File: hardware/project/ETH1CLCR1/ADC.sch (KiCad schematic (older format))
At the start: 103 parts, among them Q1101 BC847W, Q1102 BC847W, Q1103 BC847W, Q1104 BC847W, U1101 ADG419BR, U1102 ADG419BR, U1103 ADR4525BRZ, U1104 ADA4807-2ARM, U1106 AD7380, U1106 ADA4807-2ARM, U1107 ADA4807-1AKSZ-R2, U1108 LT6350, U1109 LT6350, U1110 OPA602, U1111 OPA602, U1112 PGA103, U1113 PGA103

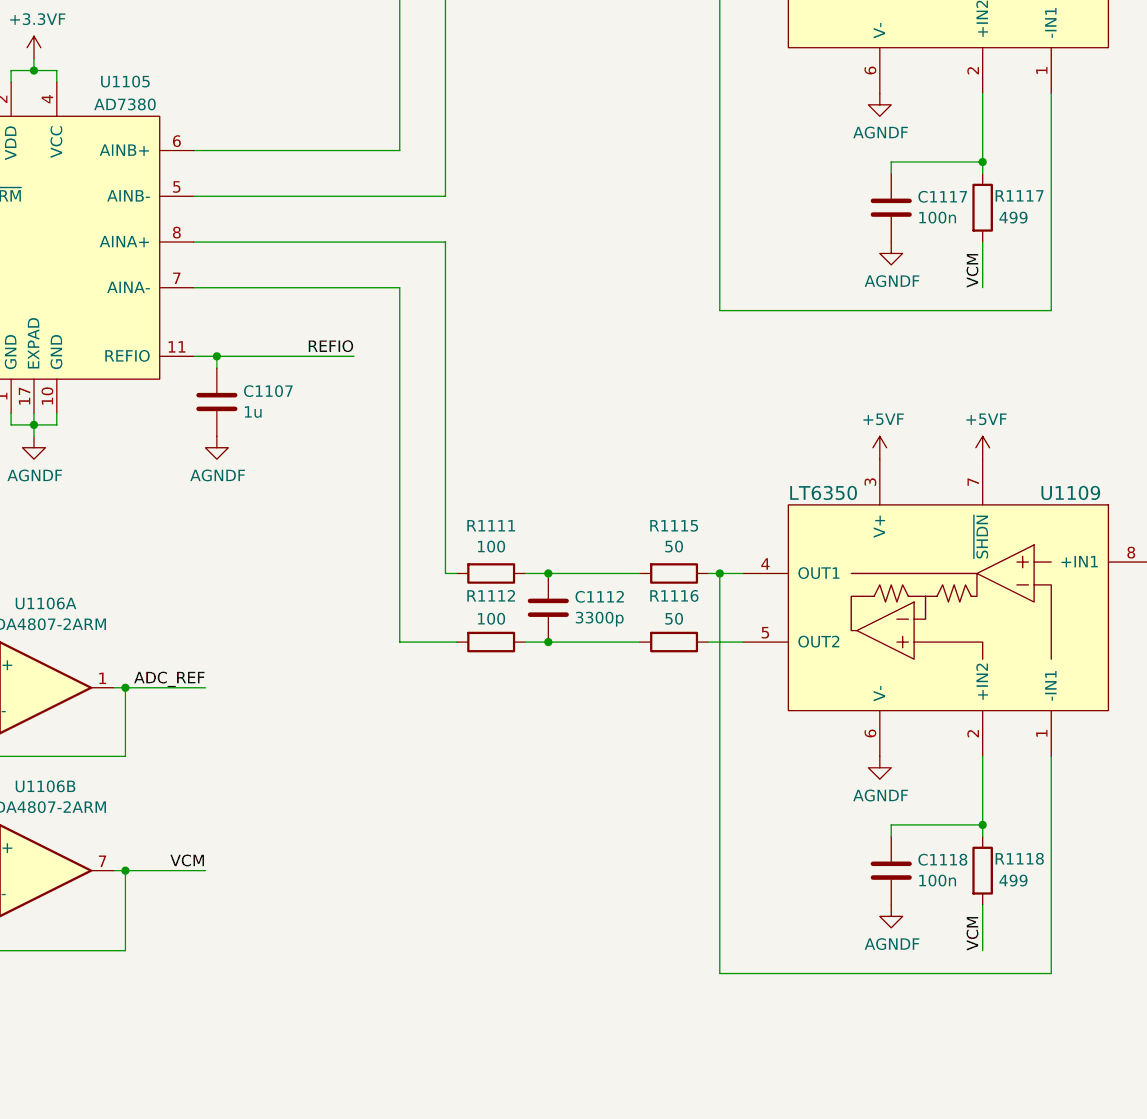
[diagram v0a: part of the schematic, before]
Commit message: PCB done.
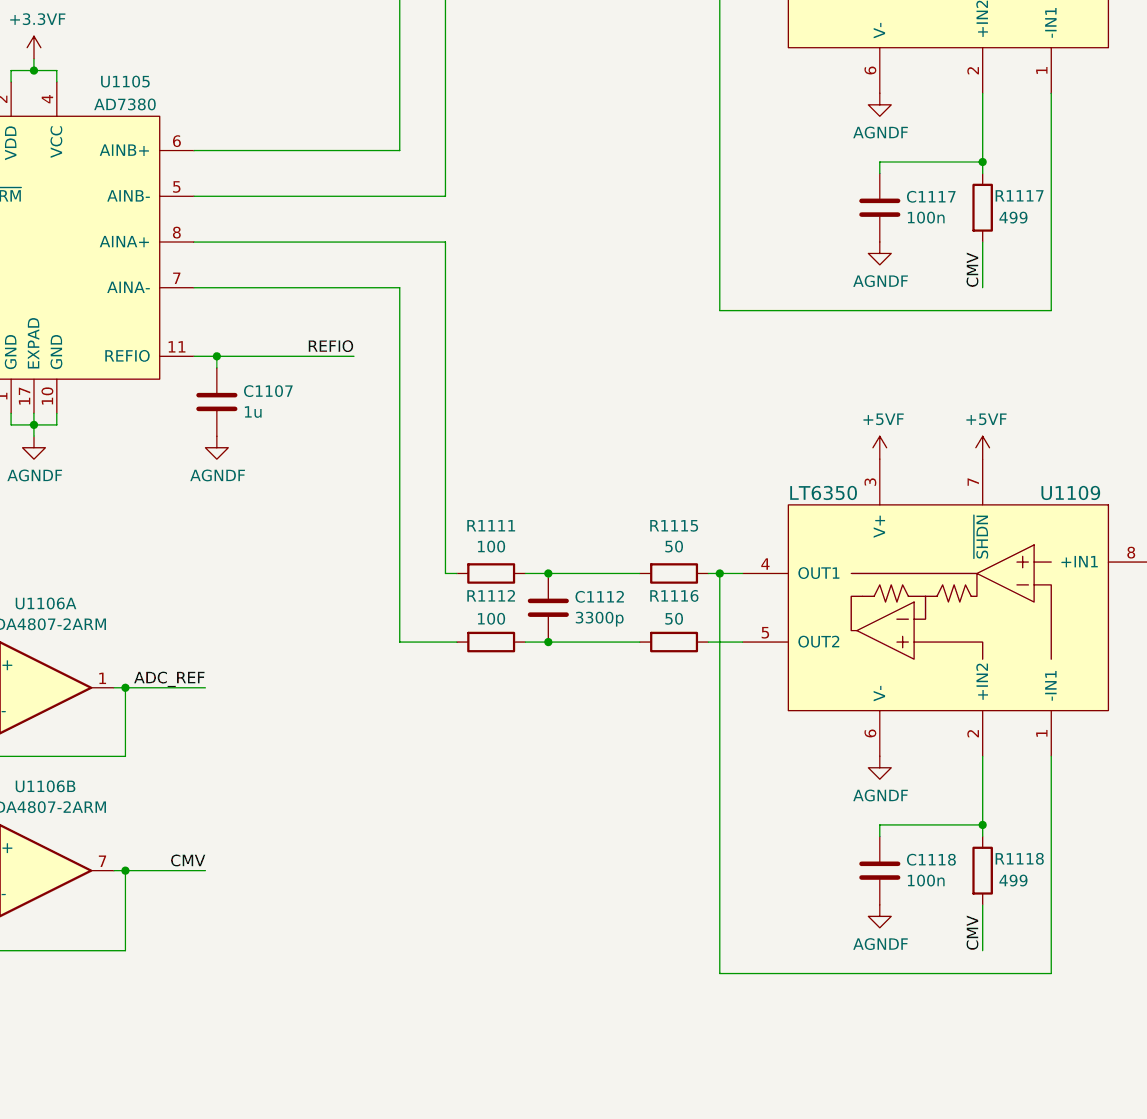
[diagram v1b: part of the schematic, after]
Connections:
- net VCM renamed CMV
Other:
- moved on the sheet: C1117, C1118
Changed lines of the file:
@@
 $EndComp
 Text Label 7600 3800 1    50   ~ 0
-VCM
+CMV
 Wire Wire Line
 	7600 3800 7600 3600
@@
 $EndComp
 Text Label 7600 6700 1    50   ~ 0
-VCM
+CMV
 Wire Wire Line
 	7600 6700 7600 6500
@@
 	2650 6250 2700 6250
 Text Label 4200 6350 2    50   ~ 0
-VCM
+CMV
 $Comp
 L Amplifier_Operational:ADA4807-2ARM U1106
@@
 L Device:C C1117
 U 1 1 5E3B70FC
-P 7200 3450
-F 0 "C1117" H 7315 3496 50  0000 L CNN
-F 1 "100n" H 7315 3405 50  0000 L CNN
-F 2 "Capacitor_SMD:C_0603_1608Metric_Pad1.05x0.95mm_HandSolder" H 7238 3300 50  0001 C CNN
-F 3 "~" H 7200 3450 50  0001 C CNN
-	1    7200 3450
+P 7150 3450
+F 0 "C1117" H 7265 3496 50  0000 L CNN
+F 1 "100n" H 7265 3405 50  0000 L CNN
+F 2 "Capacitor_SMD:C_0603_1608Metric_Pad1.05x0.95mm_HandSolder" H 7188 3300 50  0001 C CNN
+F 3 "~" H 7150 3450 50  0001 C CNN
+	1    7150 3450
 	1    0    0    -1
 $EndComp
@@
 L ETH1CLCR1:AGNDF #PWR01142
 U 1 1 5E3B7653
-P 7200 3600
-F 0 "#PWR01142" H 7200 3350 50  0001 C CNN
-F 1 "AGNDF" H 7205 3427 50  0000 C CNN
-F 2 "" H 7200 3600 50  0001 C CNN
-F 3 "" H 7200 3600 50  0001 C CNN
-	1    7200 3600
-	1    0    0    -1
-$EndComp
-Wire Wire Line
-	7200 3300 7200 3250
-Wire Wire Line
-	7200 3250 7600 3250
+P 7150 3600
+F 0 "#PWR01142" H 7150 3350 50  0001 C CNN
+F 1 "AGNDF" H 7155 3427 50  0000 C CNN
+F 2 "" H 7150 3600 50  0001 C CNN
+F 3 "" H 7150 3600 50  0001 C CNN
+	1    7150 3600
+	1    0    0    -1
+$EndComp
+Wire Wire Line
+	7150 3300 7150 3250
+Wire Wire Line
+	7150 3250 7600 3250
 Wire Wire Line
 	7600 3250 7600 3300
@@
 Wire Wire Line
 	6450 6800 6450 5050
-Wire Wire Line
-	7600 6150 7600 5850
 $Comp
 L Device:C C1118
 U 1 1 5E48656C
-P 7200 6350
-F 0 "C1118" H 7315 6396 50  0000 L CNN
-F 1 "100n" H 7315 6305 50  0000 L CNN
-F 2 "Capacitor_SMD:C_0603_1608Metric_Pad1.05x0.95mm_HandSolder" H 7238 6200 50  0001 C CNN
-F 3 "~" H 7200 6350 50  0001 C CNN
-	1    7200 6350
+P 7150 6350
+F 0 "C1118" H 7265 6396 50  0000 L CNN
+F 1 "100n" H 7265 6305 50  0000 L CNN
+F 2 "Capacitor_SMD:C_0603_1608Metric_Pad1.05x0.95mm_HandSolder" H 7188 6200 50  0001 C CNN
+F 3 "~" H 7150 6350 50  0001 C CNN
+	1    7150 6350
 	1    0    0    -1
 $EndComp
@@
 L ETH1CLCR1:AGNDF #PWR01143
 U 1 1 5E486572
-P 7200 6500
-F 0 "#PWR01143" H 7200 6250 50  0001 C CNN
-F 1 "AGNDF" H 7205 6327 50  0000 C CNN
-F 2 "" H 7200 6500 50  0001 C CNN
-F 3 "" H 7200 6500 50  0001 C CNN
-	1    7200 6500
-	1    0    0    -1
-$EndComp
-Wire Wire Line
-	7200 6200 7200 6150
-Wire Wire Line
-	7200 6150 7600 6150
-Wire Wire Line
-	7600 6200 7600 6150
-Connection ~ 7600 6150
+P 7150 6500
+F 0 "#PWR01143" H 7150 6250 50  0001 C CNN
+F 1 "AGNDF" H 7155 6327 50  0000 C CNN
+F 2 "" H 7150 6500 50  0001 C CNN
+F 3 "" H 7150 6500 50  0001 C CNN
+	1    7150 6500
+	1    0    0    -1
+$EndComp
+Wire Wire Line
+	7150 6200 7150 6150
 Connection ~ 6450 5050
 Wire Wire Line
@@
 Wire Wire Line
 	1950 3800 2000 3800
+Wire Wire Line
+	7600 5850 7600 6150
+Wire Wire Line
+	7150 6150 7600 6150
+Connection ~ 7600 6150
+Wire Wire Line
+	7600 6150 7600 6200
 $EndSCHEMATC
